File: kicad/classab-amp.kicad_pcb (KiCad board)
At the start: 2 copper layers, 87.4 x 101.9 mm, 75 parts, among them J1 SPEAKER, J3 INPUT, Q1 BC547, Q10 MJL3218C, Q11 BD140, Q12 MJL1302C, Q13 BC547, Q14 BC557, Q2 BC547, Q3 BC557, Q4 BC557, Q5 BC547, Q6 BD140, Q7 BD139, Q8 BD139, Q9 BD139

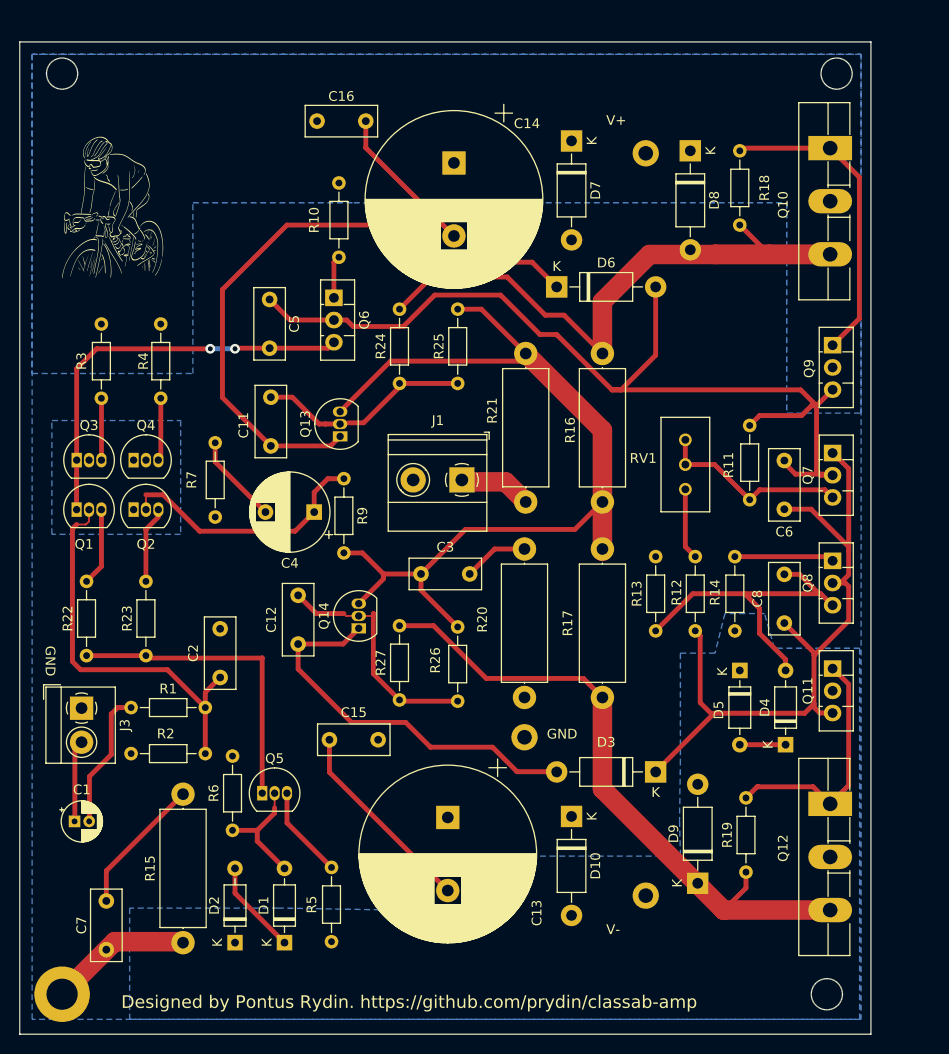
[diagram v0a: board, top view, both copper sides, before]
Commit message: Production candidate
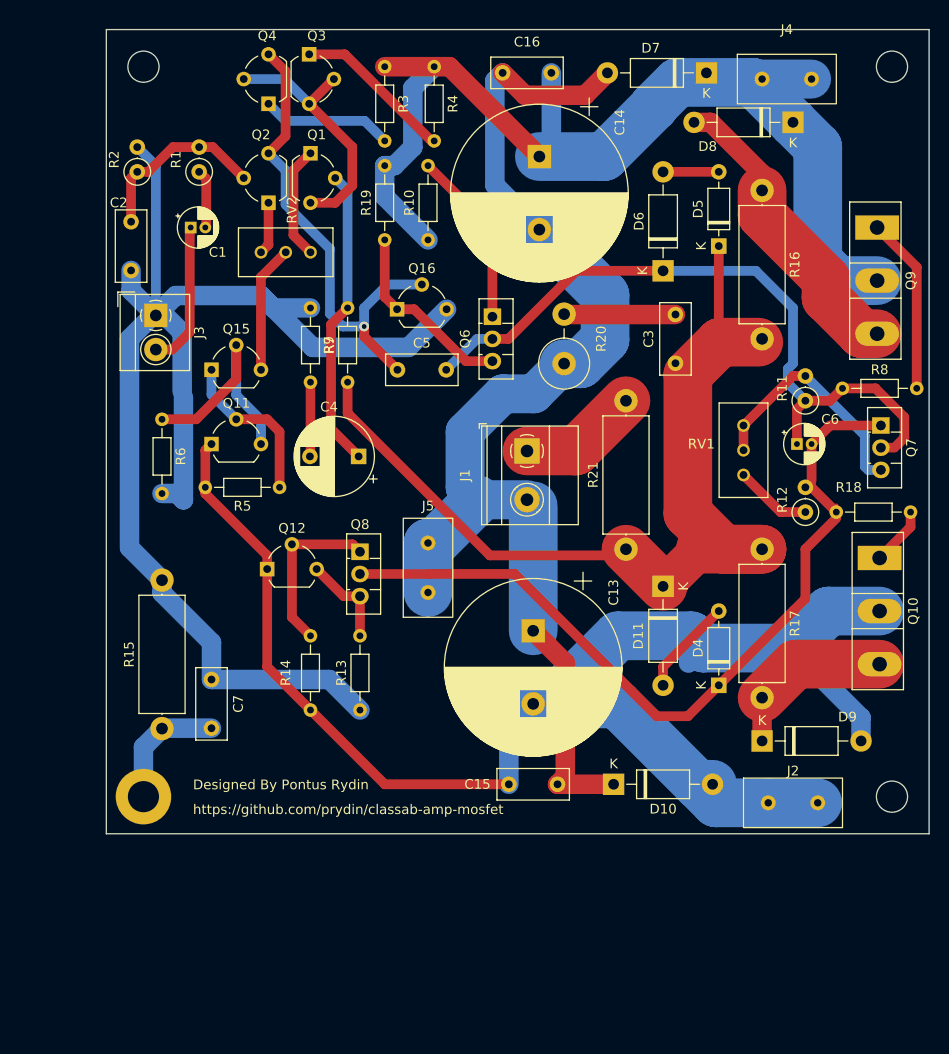
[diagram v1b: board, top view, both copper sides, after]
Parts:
- removed the ? at (247.4, 119.4)
- removed the ? at (235.0, 103.1)
- removed the ? at (247.4, 43.2)
- removed the ? at (187.5, 129.5)
- removed C11, C12: 470p, Capacitor_THT:C_Rect_L7.2mm_W3.0mm_P5.00mm_FKS2_FKP2_MKS2_MKP2
- removed C8: 4.7n, Capacitor_THT:C_Rect_L7.2mm_W3.0mm_P5.00mm_FKS2_FKP2_MKS2_MKP2
- removed D1, D2: 1N4148, Diode_THT:D_DO-35_SOD27_P7.62mm_Horizontal
- removed D3: 1N4004, Diode_THT:D_DO-41_SOD81_P10.16mm_Horizontal
- removed PIC1: LOGO, LOGO
- removed Q13, Q5: BC547, Package_TO_SOT_THT:TO-92_Inline
- removed Q14: BC557, Package_TO_SOT_THT:TO-92_Inline
- removed R22, R23: 150, Resistor_THT:R_Axial_DIN0204_L3.6mm_D1.6mm_P7.62mm_Horizontal
- removed R24, R27: 1k, Resistor_THT:R_Axial_DIN0204_L3.6mm_D1.6mm_P7.62mm_Horizontal
- removed R25, R26: 8.2k, Resistor_THT:R_Axial_DIN0204_L3.6mm_D1.6mm_P7.62mm_Horizontal
- removed the REF** at (268.0, 35.0)
- removed the REF** at (267.0, 129.5)
- removed the REF** at (188.5, 35.0)
- added ?: , , F.Cu at (195.8, 109.2)
- added D11: 1N5919, Diode_THT:D_DO-41_SOD81_P10.16mm_Horizontal, F.Cu at (250.2, 87.6)
- added J2: ~, footprints:Spade Connector, F.Cu at (263.5, 104.8)
- added J4: ~, footprints:Spade Connector, F.Cu at (262.9, 30.5)
- added J5: ~, footprints:Spade Connector, F.Cu at (221.0, 85.7)
- added Q15: 2N5551, Package_TO_SOT_THT:TO-92_Wide, F.Cu at (203.8, 65.4)
- added Q16: 2N5401, Package_TO_SOT_THT:TO-92_Wide, F.Cu at (222.9, 59.2)
- added R8: 330, Resistor_THT:R_Axial_DIN0204_L3.6mm_D1.6mm_P7.62mm_Horizontal, F.Cu at (268.6, 67.3)
- added REF**: MountingHole_3.2mm_M3, MountingHole:MountingHole_3.2mm_M3, F.Cu at (273.7, 109.2)
- added REF**: MountingHole_3.2mm_M3, MountingHole:MountingHole_3.2mm_M3, F.Cu at (196.8, 34.3)
- added REF**: MountingHole_3.2mm_M3, MountingHole:MountingHole_3.2mm_M3, F.Cu at (273.7, 34.3)
- added RV2: 300, footprints:TRIM_T93YA103KT20, F.Cu at (211.5, 53.3)
- C2: value 220p -> 100p
- C5: value 50p -> 100p
- C6: value 100n -> 10u; footprint Capacitor_THT:C_Rect_L7.2mm_W3.0mm_P5.00mm_FKS2_FKP2_MKS2_MKP2 -> Capacitor_THT:CP_Radial_D4.0mm_P1.50mm
- D6: value 1N4004 -> 1N5919
- Q1, Q2: value BC547 -> 2N5551; footprint Package_TO_SOT_THT:TO-92_Inline -> Package_TO_SOT_THT:TO-92_Wide
- Q10: value MJL3218C -> IRFP9240; footprint Package_TO_SOT_THT:TO-264-3_Vertical -> Package_TO_SOT_THT:TO-247-3_Vertical
- Q11: value BD140 -> 2N5551; footprint Package_TO_SOT_THT:TO-126-3_Vertical -> Package_TO_SOT_THT:TO-92_Wide
- Q12: value MJL1302C -> 2N5551; footprint Package_TO_SOT_THT:TO-264-3_Vertical -> Package_TO_SOT_THT:TO-92_Wide
- Q3, Q4: value BC557 -> 2N5401; footprint Package_TO_SOT_THT:TO-92_Inline -> Package_TO_SOT_THT:TO-92_Wide
- Q9: value BD139 -> IRFP240; footprint Package_TO_SOT_THT:TO-126-3_Vertical -> Package_TO_SOT_THT:TO-247-3_Vertical
- R1, R2: footprint Resistor_THT:R_Axial_DIN0204_L3.6mm_D1.6mm_P7.62mm_Horizontal -> Resistor_THT:R_Axial_DIN0207_L6.3mm_D2.5mm_P2.54mm_Vertical
- R10, R14: value 150 -> 100
- R11: value 22k -> 4.7k; footprint Resistor_THT:R_Axial_DIN0204_L3.6mm_D1.6mm_P7.62mm_Horizontal -> Resistor_THT:R_Axial_DIN0207_L6.3mm_D2.5mm_P2.54mm_Vertical
- R12: value 15k -> 330; footprint Resistor_THT:R_Axial_DIN0204_L3.6mm_D1.6mm_P7.62mm_Horizontal -> Resistor_THT:R_Axial_DIN0207_L6.3mm_D2.5mm_P2.54mm_Vertical
- R16, R17: value 0.22 -> 0.33
- R18: value 1.5k -> 330
- R19: value 1.5k -> 1k
- R20: footprint Resistor_THT:R_Axial_DIN0414_L11.9mm_D4.5mm_P15.24mm_Horizontal -> Resistor_THT:R_Axial_DIN0516_L15.5mm_D5.0mm_P5.08mm_Vertical
- R3, R4, R5: value 1k -> 470
- R6: value 10k -> 4.7k
- R7: value 1k -> 2.2k
- R9: value 22k -> 47k
- RV1: value 10k -> 300
- moved R19 81.4 mm to (221.6, 44.5), turned to -90 degrees
- moved Q11 67.8 mm to (203.8, 73.0), turned to 0 degrees
- moved Q12 62.6 mm to (209.6, 85.9), turned to 0 degrees
- moved C1 62.1 mm to (201.7, 50.8)
- moved R2 60.1 mm to (196.2, 45.1), turned to 90 degrees
- moved R1 55.4 mm to (202.6, 45.1), turned to 90 degrees
- moved Q8 48.5 mm to (219.1, 84.1)
- moved Q3 48.0 mm to (213.9, 33.0), turned to -90 degrees
- moved C2 47.7 mm to (195.6, 50.2), turned to -90 degrees
- moved R14 44.3 mm to (214.0, 92.7)
- moved Q1 43.7 mm to (214.0, 43.2), turned to -90 degrees
- moved D5 43.6 mm to (255.9, 52.7), turned to 90 degrees
- moved R6 42.8 mm to (198.8, 70.5), turned to -90 degrees
- moved Q10 42.4 mm to (272.4, 84.7)
- moved J3 41.0 mm to (198.1, 59.8)
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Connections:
- net /INPUT renamed Net-(J3-Pin_2)
- C13 pad 1: GND -> PWRGND
- C14 pad 2: GND -> PWRGND
- C15 pad 2: GND -> PWRGND
- C16 pad 1: GND -> PWRGND
- C2 pad 1: Net-(Q1-B) -> Net-(Q2-B)
- C3 pad 1: Net-(Q13-E) -> Net-(D11-K)
- C4 pad 1: Net-(Q2-B) -> Net-(Q1-B)
- C5 pad 1: Net-(Q1-C) -> Net-(Q16-B)
- C5 pad 2: Net-(D6-A) -> Net-(D6-K)
- C6 pad 1: Net-(D6-A) -> Net-(D6-K)
- C6 pad 2: Net-(D3-K) -> Net-(D4-K)
- D10 pad 1: GND -> PWRGND
- D4 pad 2: Net-(D4-A) -> Net-(D11-A)
- D5 pad 1: B- -> Net-(D11-K)
- D5 pad 2: Net-(D4-K) -> Net-(D5-A)
- D6 pad 2: Net-(D6-A) -> Net-(D5-A)
- D7 pad 2: GND -> PWRGND
- J1 pad 2: GND -> PWRGND
- Q1 pad 1: Net-(Q1-C) -> Net-(Q1-E)
- Q1 pad 3: Net-(Q1-E) -> /LTP COM
- Q10 pad 1: Net-(Q10-B) -> Net-(Q10-G)
- Q10 pad 2: B+ -> B-
- Q10 pad 3: Net-(D8-A) -> Net-(D9-K)
- Q11 pad 1: Net-(Q11-E) -> B-
- Q11 pad 2: B- -> Net-(Q11-B)
- Q11 pad 3: Net-(D3-K) -> Net-(Q11-C)
- Q12 pad 1: Net-(Q11-E) -> B-
- Q12 pad 2: B- -> Net-(Q12-B)
- Q12 pad 3: Net-(D9-K) -> Net-(Q12-C)
- Q2 pad 1: /LTP COM -> Net-(Q2-E)
- Q2 pad 3: Net-(Q2-E) -> Net-(Q16-B)
- Q3 pad 1: Net-(Q1-C) -> Net-(Q3-E)
- Q3 pad 3: Net-(Q3-E) -> /LTP COM
- Q4 pad 1: /LTP COM -> Net-(Q4-E)
- Q4 pad 3: Net-(Q4-E) -> Net-(Q16-B)
- Q6 pad 2: Net-(D6-A) -> Net-(D6-K)
- Q6 pad 3: Net-(Q1-C) -> Net-(Q16-E)
- Q7 pad 1: Net-(D3-K) -> Net-(D4-K)
- Q7 pad 2: Net-(D6-A) -> Net-(D6-K)
- Q8 pad 1: Net-(Q8-E) -> Net-(Q12-B)
- Q8 pad 2: Net-(D3-K) -> Net-(D4-K)
- Q8 pad 3: Net-(D4-A) -> Net-(Q12-C)
- Q9 pad 1: Net-(Q10-B) -> Net-(Q9-G)
- Q9 pad 3: Net-(D6-A) -> Net-(D8-A)
- R1 pad 2: Net-(Q1-B) -> Net-(Q2-B)
- R11 pad 1: Net-(D6-A) -> Net-(D6-K)
- R12 pad 2: Net-(D3-K) -> Net-(D4-K)
- R13 pad 1: Net-(D4-A) -> Net-(Q12-C)
- R14 pad 1: Net-(Q8-E) -> Net-(Q12-B)
- R16 pad 2: Net-(Q13-E) -> Net-(D11-K)
- R17 pad 1: Net-(Q13-E) -> Net-(D11-K)
- R18 pad 1: Net-(Q10-B) -> Net-(D4-K)
- R18 pad 2: Net-(D8-A) -> Net-(Q10-G)
- R19 pad 1: Net-(D9-K) -> B+
- R19 pad 2: Net-(Q11-E) -> Net-(Q16-E)
- R2 pad 1: Net-(Q1-B) -> Net-(Q2-B)
- R20 pad 1: Net-(C3-Pad2) -> PWRGND
- R20 pad 2: GND -> Net-(C3-Pad2)
- R21 pad 1: Net-(Q13-E) -> Net-(D11-K)
- R3 pad 2: Net-(Q3-E) -> Net-(Q4-E)
- R4 pad 2: Net-(Q4-E) -> Net-(Q3-E)
- R5 pad 1: Net-(Q5-E) -> Net-(Q11-B)
- R6 pad 1: Net-(D1-A) -> Net-(Q11-C)
- R9 pad 1: Net-(Q2-B) -> Net-(Q1-B)
- R9 pad 2: Net-(Q13-E) -> Net-(D11-K)
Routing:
- net B-: track 20.5 -> 158.6 mm
- net PWRGND: track 0.00 -> 123.9 mm
- net GND: track 29.8 -> 145.6 mm
- net B+: track 0.00 -> 109.3 mm
- net Net-(D6-A): track 100.5 -> 0.00 mm
- net Net-(D11-K): track 0.00 -> 98.9 mm
- net Net-(Q13-E): track 95.7 -> 0.00 mm
- net Net-(D4-K): track 4.70 -> 85.4 mm
- net Net-(D3-K): track 74.3 -> 0.00 mm
- net Net-(Q16-B): track 0.00 -> 49.4 mm, vias 0 -> 1
- net Net-(D9-K): track 66.6 -> 17.9 mm
- net Net-(D8-A): track 79.4 -> 31.4 mm
- net Net-(Q1-C): track 47.6 -> 0.00 mm, vias 2 -> 0
- net Net-(D3-A): track 40.4 -> 0.00 mm
- net Net-(D4-A): track 34.0 -> 0.00 mm
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- removed copper zone on B.Cu, net /LTP COM
- removed copper zone on B.Cu, net B+
- removed copper zone on B.Cu, net B-
- removed copper zone on B.Cu, net GND
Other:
- board size 87.4 x 101.9 mm -> 84.5 x 82.5 mm
- board text added: "Designed By Pontus Rydin"
- board text added: "https://github.com/prydin/classab-amp-mosfet"
- board text removed: "Designed by Pontus Rydin. https://github.com/prydin/classab-amp"
- board text removed: "GND"
- board text removed: "V+"
- board text removed: "V-"
